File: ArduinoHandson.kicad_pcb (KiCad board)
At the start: 2 copper layers, 34.3 x 64.8 mm, 19 parts, among them IC1 ATMEGA328-P, P2 USB micro, P3 Power, P4 Digital2, P5 Analog, P6 Digital1, SW1 Reset, U1 FT232RL, X1 CRYSTAL

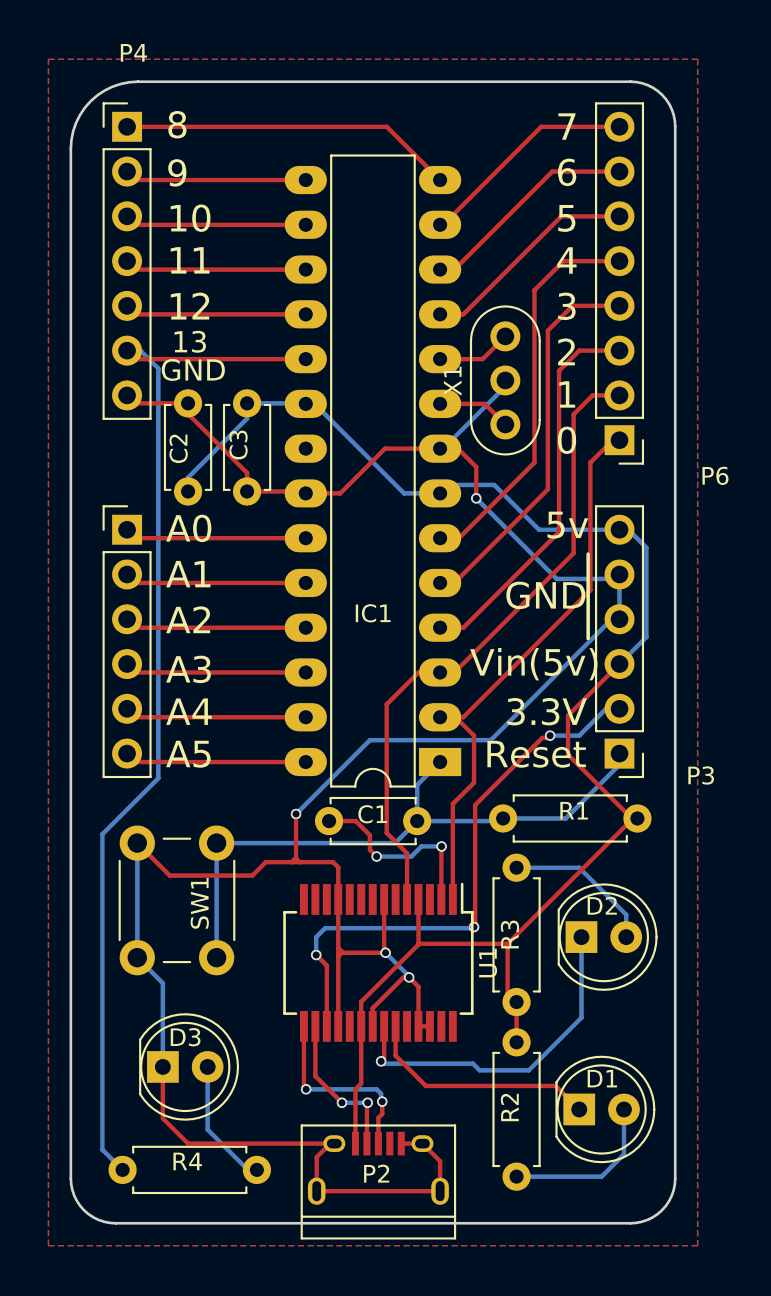
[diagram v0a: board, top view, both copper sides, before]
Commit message: 回路図+配線図完成
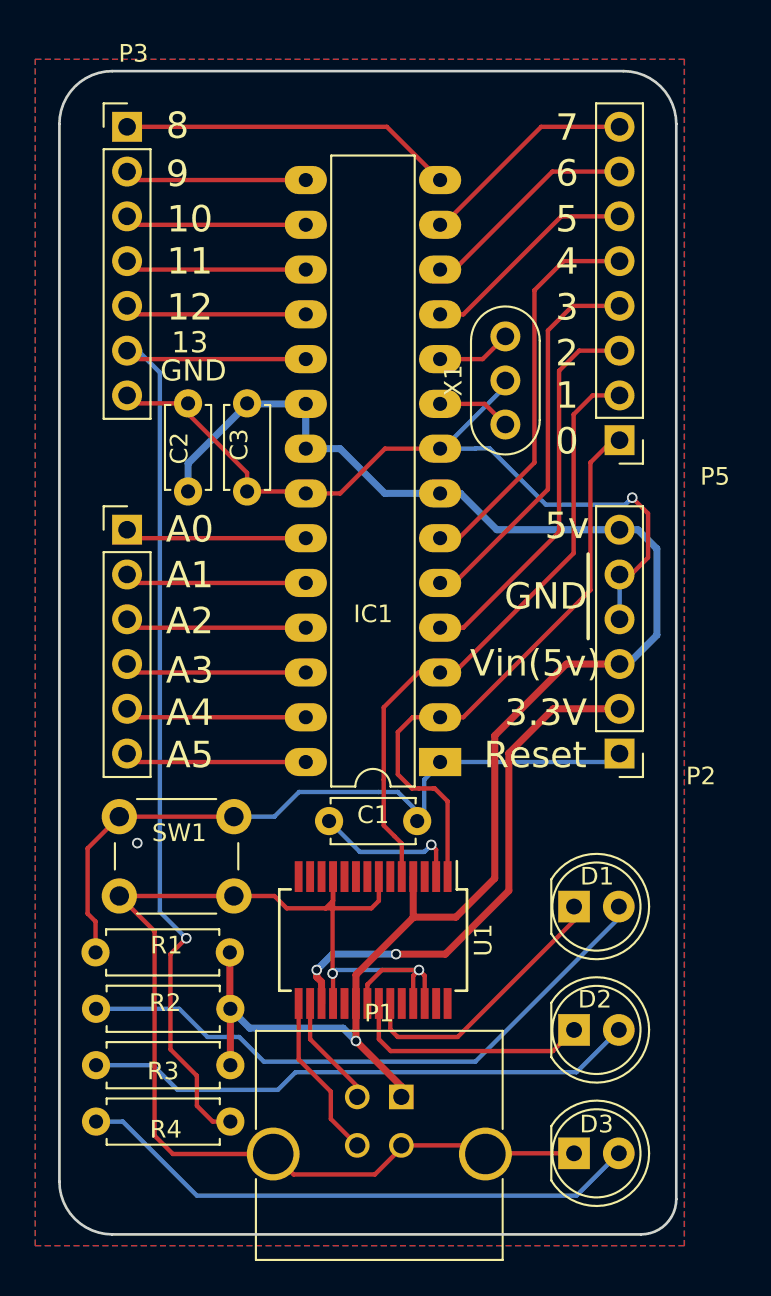
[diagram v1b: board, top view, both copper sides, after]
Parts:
- removed the P2 at (54.9, 94.6)
- added P1: USB_B, Connect:USB_B_MUSB_Straight, F.Cu at (56.2, 90.6)
- SW1: value Reset -> SW_PUSH
- moved R1 24.3 mm to (38.9, 82.4)
- moved D3 23.8 mm to (66.0, 93.8)
- moved R3 16.6 mm to (46.5, 88.8), turned to 180 degrees
- moved R2 16.3 mm to (46.5, 85.6), turned to 180 degrees
- moved D1 11.5 mm to (66.0, 79.8)
- moved R4 6.70 mm to (46.5, 92.0), turned to 180 degrees
- moved SW1 5.72 mm to (40.2, 74.7), turned to 0 degrees
- moved D2 5.28 mm to (66.0, 86.8)
- moved U1 1.33 mm to (54.6, 81.7)
- renumbered P3 to P2, P4 to P3, P5 to P4, P6 to P5
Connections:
- IC1 pad 21: Net-(IC1-Pad21) -> +5V
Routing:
- net Net-(D1-Pad2): track 9.16 -> 34.9 mm
- net Net-(D3-Pad2): track 7.30 -> 32.4 mm
- net Net-(D2-Pad2): track 8.60 -> 31.6 mm
- net GND: track 149.0 -> 129.8 mm, vias 5 -> 3
- net +5V: track 88.4 -> 96.3 mm, vias 0 -> 1
- net /Reset: track 35.7 -> 42.1 mm
- net Net-(D2-Pad1): track 19.4 -> 13.9 mm, vias 1 -> 0
- net Net-(C1-Pad1): track 11.0 -> 8.60 mm, vias 2 -> 1
- net /D-: track 8.75 -> 6.41 mm, vias 2 -> 0
- net Net-(D1-Pad1): track 13.3 -> 15.6 mm
- net +3V3: track 31.9 -> 29.9 mm, vias 3 -> 2
- net /D0: track 34.2 -> 35.8 mm
- net /D+: track 10.9 -> 9.43 mm, vias 2 -> 0
- net /D1: track 36.6 -> 35.3 mm
- net /D13: track 59.8 -> 59.0 mm, vias 0 -> 1
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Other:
- board size 34.3 x 64.8 mm -> 35 x 66 mm
- net class Power added: clearance 0.2, trace_width 0.4, via_dia 0.6, via_drill 0.4
